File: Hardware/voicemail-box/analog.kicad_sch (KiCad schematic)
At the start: 18 parts, among them J601 AudioJack3_Ground, J602 AudioJack4_SwitchT1, U601 TLV320AIC3104

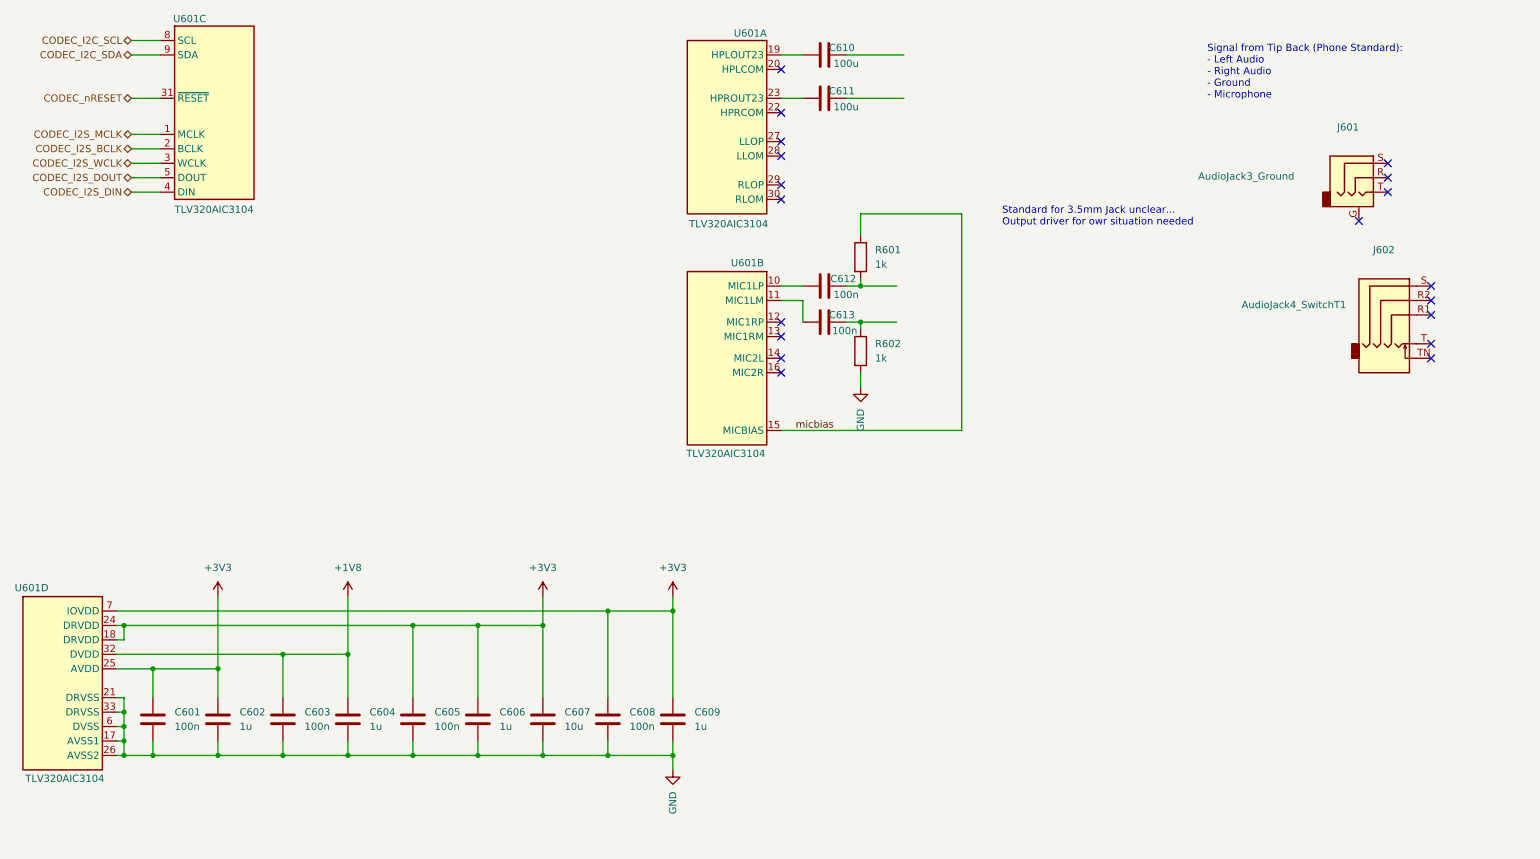
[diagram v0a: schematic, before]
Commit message: schema review
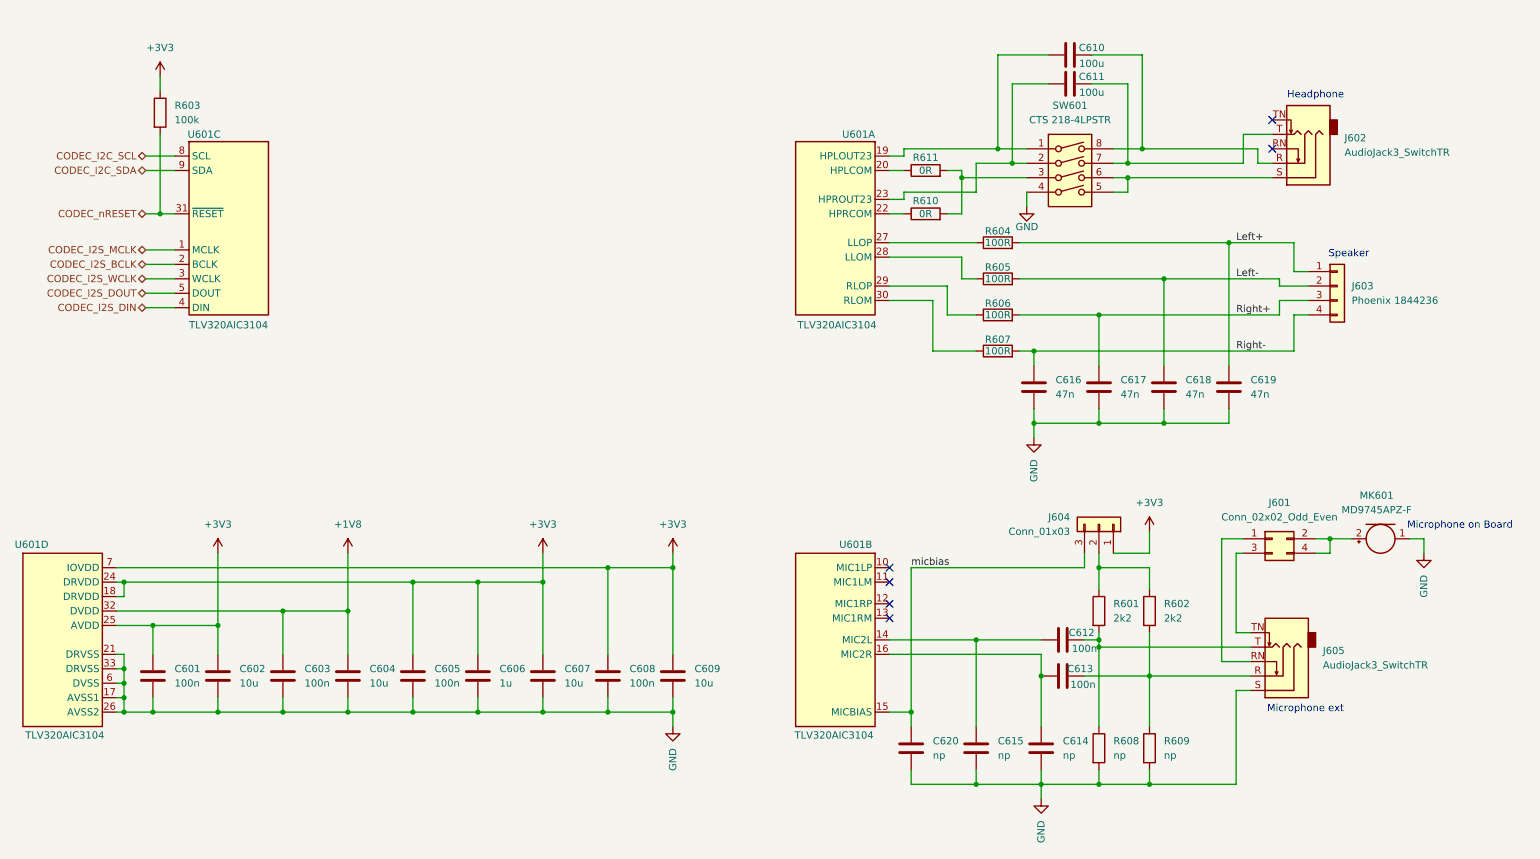
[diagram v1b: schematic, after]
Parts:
- removed J601: AudioJack3_Ground, Connector_Audio:Jack_3.5mm_CUI_SJ-3524-SMT_Horizontal, symbol Connector_Audio:AudioJack3_Ground
- removed J602: AudioJack4_SwitchT1, Connector_Audio:Jack_3.5mm_CUI_SJ1-3515N_Horizontal, symbol Connector_Audio:AudioJack4_SwitchT1
- added C614, C615, C620: np, Capacitor_SMD:C_0603_1608Metric_Pad1.08x0.95mm_HandSolder, symbol Device:C
- added C616, C617, C618, C619: 47n, Capacitor_SMD:C_0603_1608Metric_Pad1.08x0.95mm_HandSolder, symbol Device:C
- added J601: Conn_02x02_Odd_Even, Connector_PinHeader_2.54mm:PinHeader_2x02_P2.54mm_Vertical, symbol Connector_Generic:Conn_02x02_Odd_Even
- added J602, J605: AudioJack3_SwitchTR, Connector_Audio:Jack_3.5mm_CUI_SJ2-3593D-SMT_Horizontal, symbol Connector_Audio:AudioJack3_SwitchTR
- added J603: Phoenix 1844236, Connector_Phoenix_MC:PhoenixContact_MC_1,5_4-G-3.5_1x04_P3.50mm_Horizontal, symbol Connector_Generic:Conn_01x04
- added J604: Conn_01x03, Connector_PinHeader_2.54mm:PinHeader_1x03_P2.54mm_Vertical, symbol Connector_Generic:Conn_01x03
- added MK601: MD9745APZ-F, Connector_PinHeader_2.54mm:PinHeader_1x02_P2.54mm_Vertical, symbol Device:Microphone
- added R603: 100k, Resistor_SMD:R_0603_1608Metric_Pad0.98x0.95mm_HandSolder, symbol Device:R
- added R604, R605, R606, R607: 100R, Resistor_SMD:R_0603_1608Metric_Pad0.98x0.95mm_HandSolder, symbol Device:R
- added R608, R609: np, Resistor_SMD:R_0603_1608Metric_Pad0.98x0.95mm_HandSolder, symbol Device:R
- added R610, R611: 0R, Resistor_SMD:R_0603_1608Metric_Pad0.98x0.95mm_HandSolder, symbol Device:R
- added SW601: CTS 218-4LPSTR, Package_SO:SSOP-8_3.9x5.05mm_P1.27mm, symbol Switch:SW_DIP_x04
- C602, C604, C609: value 1u -> 10u
- R601, R602: value 1k -> 2k2; footprint PCM_4ms_Resistor:R_0603 -> Resistor_SMD:R_0603_1608Metric_Pad0.98x0.95mm_HandSolder
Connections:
- net +3V3: now also J604.1 (Pin_1), R603.1
- net CODEC_nRESET: now also R603.2
- net GND: now also C614.2, C615.2, C616.2, C617.2, C618.2, C619.2, C620.2, J605.S, MK601.1 (-), R608.2, R609.2, SW601.4; no longer R602.2
- net micbias: now also C620.1, J604.3 (Pin_3); no longer R601.1
- net at C611.1, U601.23 (HPROUT23): now also SW601.2
- net at C611.2: now also J602.T, SW601.7
- net at C610.1, U601.19 (HPLOUT23): now also SW601.1
- net at U601.20 (HPLCOM): now also R611.1
- net at U601.22 (HPRCOM): now also R610.1
- net at U601.27 (LLOP): now also R604.1
- net at U601.28 (LLOM): now also R605.1
- net at U601.29 (RLOP): now also R606.1
- net at U601.30 (RLOM): now also R607.1
- net at C612.2, R601.2: now also J605.T, R608.1
- net at C613.1: now also U601.16 (MIC2R), C614.1; no longer U601.11 (MIC1LM)
- net at C613.2: now also R602.2, J605.R, R609.1; no longer R602.1
- net at U601.10 (MIC1LP): no longer C612.1
- net at U601.14 (MIC2L): now also C612.1, C615.1
- net at C610.2: now also J602.R, SW601.8
- new net: R610.2, R611.2, SW601.3
- new net: J602.S, SW601.5, SW601.6
- new net: J601.2 (Pin_2), J601.4 (Pin_4), MK601.2 (+)
- new net: J604.2 (Pin_2), R601.1, R602.1
- new net: J601.1 (Pin_1), J605.RN
- new net: J601.3 (Pin_3), J605.TN
- new net Left+: C619.1, J603.1 (Pin_1), R604.2
- new net Left-: C618.1, J603.2 (Pin_2), R605.2
- new net Right+: C617.1, J603.3 (Pin_3), R606.2
- new net Right-: C616.1, J603.4 (Pin_4), R607.2
- no-connect marks 19 -> 6
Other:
- note added: "Headphone"
- note added: "Microphone ext"
- note added: "Microphone on Board"
- note added: "Speaker"
- note removed: "Signal from Tip Back (Phone Standard): - Left Audio - Right Audio - Ground - Microphone"
- note removed: "Standard for 3.5mm Jack unclear... Output driver for owr situation needed"
- moved on the sheet: C601, C602, C603, C604, C605, C606, C607, C608, C609, C610, C611, C612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
